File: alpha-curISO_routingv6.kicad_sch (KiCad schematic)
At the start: 27 parts, among them J2 SWD, Q1 2N2222, U1 RP2040, U5 74AHCT1G125

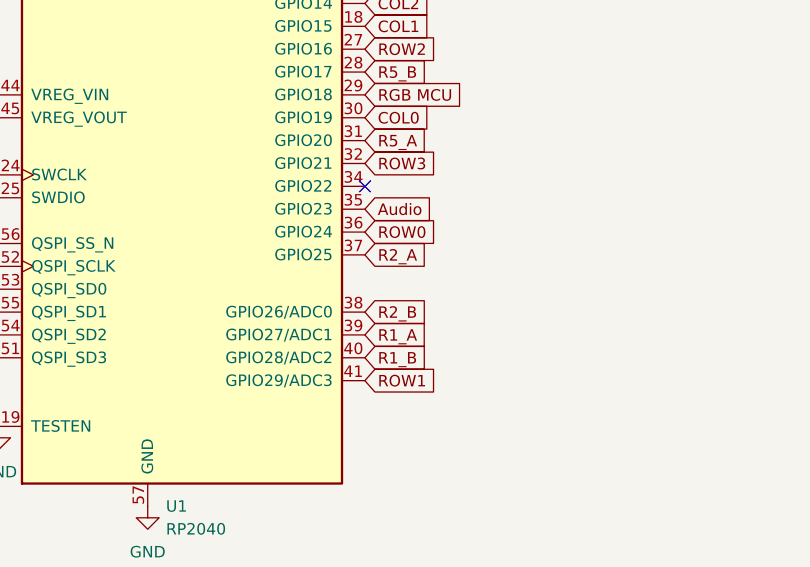
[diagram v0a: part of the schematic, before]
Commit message: changed nets a bit
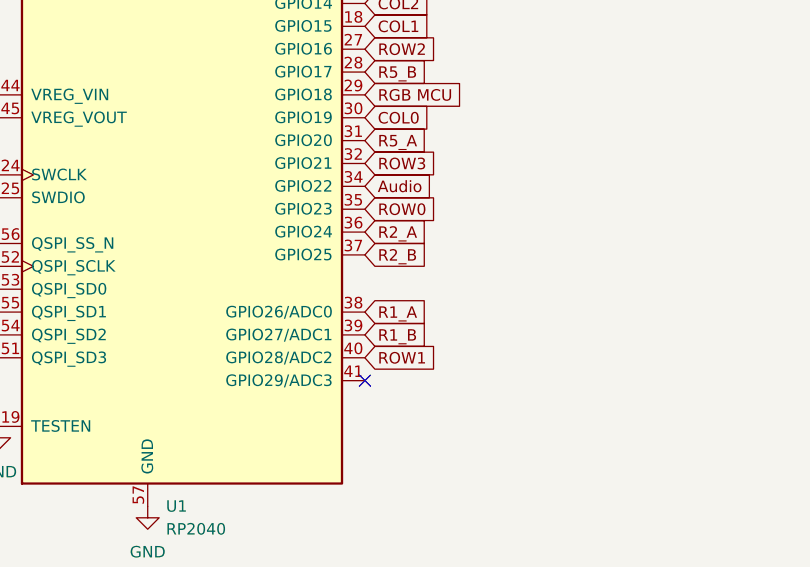
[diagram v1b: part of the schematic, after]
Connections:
- net Audio: now also U1.34 (GPIO22); no longer U1.35 (GPIO23)
- net R1_A: now also U1.38 (GPIO26/ADC0); no longer U1.39 (GPIO27/ADC1)
- net R1_B: now also U1.39 (GPIO27/ADC1); no longer U1.40 (GPIO28/ADC2)
- net R2_A: now also U1.36 (GPIO24); no longer U1.37 (GPIO25)
- net R2_B: now also U1.37 (GPIO25); no longer U1.38 (GPIO26/ADC0)
- net ROW0: now also U1.35 (GPIO23); no longer U1.36 (GPIO24)
- net ROW1: now also U1.40 (GPIO28/ADC2); no longer U1.41 (GPIO29/ADC3)
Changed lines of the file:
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@@
   (junction (at 302.895 170.18) (diameter 0) (color 0 0 0 0)
   )
-  (no_connect (at 80.01 92.71))
+  (no_connect (at 80.01 114.3))
   (wire (pts (xy 298.45 243.84) (xy 315.595 243.84))
     (stroke (width 0) (type default) (color 0 0 0 0))
@@
     )
   )
-  (global_label "R2_B" (shape input) (at 80.01 106.68 0) (fields_autoplaced)
-    (effects (font (size 1.27 1.27)) (justify left))
-    (property "Intersheet References" "${INTERSHEET_REFS}" (id 0) (at 87.1402 106.7594 0)
+  (global_label "R2_B" (shape input) (at 80.01 100.33 0) (fields_autoplaced)
+    (effects (font (size 1.27 1.27)) (justify left))
+    (property "Intersheet References" "${INTERSHEET_REFS}" (id 0) (at 87.1402 100.4094 0)
       (effects (font (size 1.27 1.27)) (justify left) hide)
     )
@@
     )
   )
-  (global_label "ROW1" (shape input) (at 80.01 114.3 0) (fields_autoplaced)
-    (effects (font (size 1.27 1.27)) (justify left))
-    (property "Intersheet References" "${INTERSHEET_REFS}" (id 0) (at 87.6845 114.3794 0)
+  (global_label "ROW1" (shape input) (at 80.01 111.76 0) (fields_autoplaced)
+    (effects (font (size 1.27 1.27)) (justify left))
+    (property "Intersheet References" "${INTERSHEET_REFS}" (id 0) (at 87.6845 111.8394 0)
       (effects (font (size 1.27 1.27)) (justify left) hide)
     )
@@
     )
   )
-  (global_label "R2_A" (shape input) (at 80.01 100.33 0) (fields_autoplaced)
-    (effects (font (size 1.27 1.27)) (justify left))
-    (property "Intersheet References" "${INTERSHEET_REFS}" (id 0) (at 86.9588 100.4094 0)
+  (global_label "R2_A" (shape input) (at 80.01 97.79 0) (fields_autoplaced)
+    (effects (font (size 1.27 1.27)) (justify left))
+    (property "Intersheet References" "${INTERSHEET_REFS}" (id 0) (at 86.9588 97.8694 0)
       (effects (font (size 1.27 1.27)) (justify left) hide)
     )
@@
     )
   )
-  (global_label "ROW0" (shape input) (at 80.01 97.79 0) (fields_autoplaced)
-    (effects (font (size 1.27 1.27)) (justify left))
-    (property "Intersheet References" "${INTERSHEET_REFS}" (id 0) (at 87.6845 97.8694 0)
+  (global_label "ROW0" (shape input) (at 80.01 95.25 0) (fields_autoplaced)
+    (effects (font (size 1.27 1.27)) (justify left))
+    (property "Intersheet References" "${INTERSHEET_REFS}" (id 0) (at 87.6845 95.3294 0)
       (effects (font (size 1.27 1.27)) (justify left) hide)
     )
@@
     )
   )
-  (global_label "Audio" (shape input) (at 80.01 95.25 0) (fields_autoplaced)
-    (effects (font (size 1.27 1.27)) (justify left))
-    (property "Intersheet References" "${INTERSHEET_REFS}" (id 0) (at 87.5636 95.3294 0)
+  (global_label "Audio" (shape input) (at 80.01 92.71 0) (fields_autoplaced)
+    (effects (font (size 1.27 1.27)) (justify left))
+    (property "Intersheet References" "${INTERSHEET_REFS}" (id 0) (at 87.5636 92.7894 0)
       (effects (font (size 1.27 1.27)) (justify left) hide)
     )
@@
     )
   )
-  (global_label "R1_A" (shape input) (at 80.01 109.22 0) (fields_autoplaced)
-    (effects (font (size 1.27 1.27)) (justify left))
-    (property "Intersheet References" "${INTERSHEET_REFS}" (id 0) (at 86.9588 109.2994 0)
+  (global_label "R1_A" (shape input) (at 80.01 106.68 0) (fields_autoplaced)
+    (effects (font (size 1.27 1.27)) (justify left))
+    (property "Intersheet References" "${INTERSHEET_REFS}" (id 0) (at 86.9588 106.7594 0)
       (effects (font (size 1.27 1.27)) (justify left) hide)
     )
@@
     )
   )
-  (global_label "R1_B" (shape input) (at 80.01 111.76 0) (fields_autoplaced)
-    (effects (font (size 1.27 1.27)) (justify left))
-    (property "Intersheet References" "${INTERSHEET_REFS}" (id 0) (at 87.1402 111.8394 0)
-      (effects (font (size 1.27 1.27)) (justify left) hide)
-    )
+  (global_label "R1_B" (shape input) (at 80.01 109.22 0) (fields_autoplaced)
+    (effects (font (size 1.27 1.27)) (justify left))
+    (property "Intersheet References" "${INTERSHEET_REFS}" (id 0) (at 87.1402 109.2994 0)
+      (effects (font (size 1.27 1.27)) (justify left) hide)
+    )
